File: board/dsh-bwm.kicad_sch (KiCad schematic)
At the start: 17 parts, among them IC2 MAX485CSA+T, K1 833H-1C-C-24VDC, K2 833H-1C-C-24VDC, K3 833H-1C-C-24VDC, K4 833H-1C-C-24VDC, Q1 IRLB8721PBF, SW1 BOOTSEL, SW2 SW_DIP_x09, U1 RP2040_Stamp

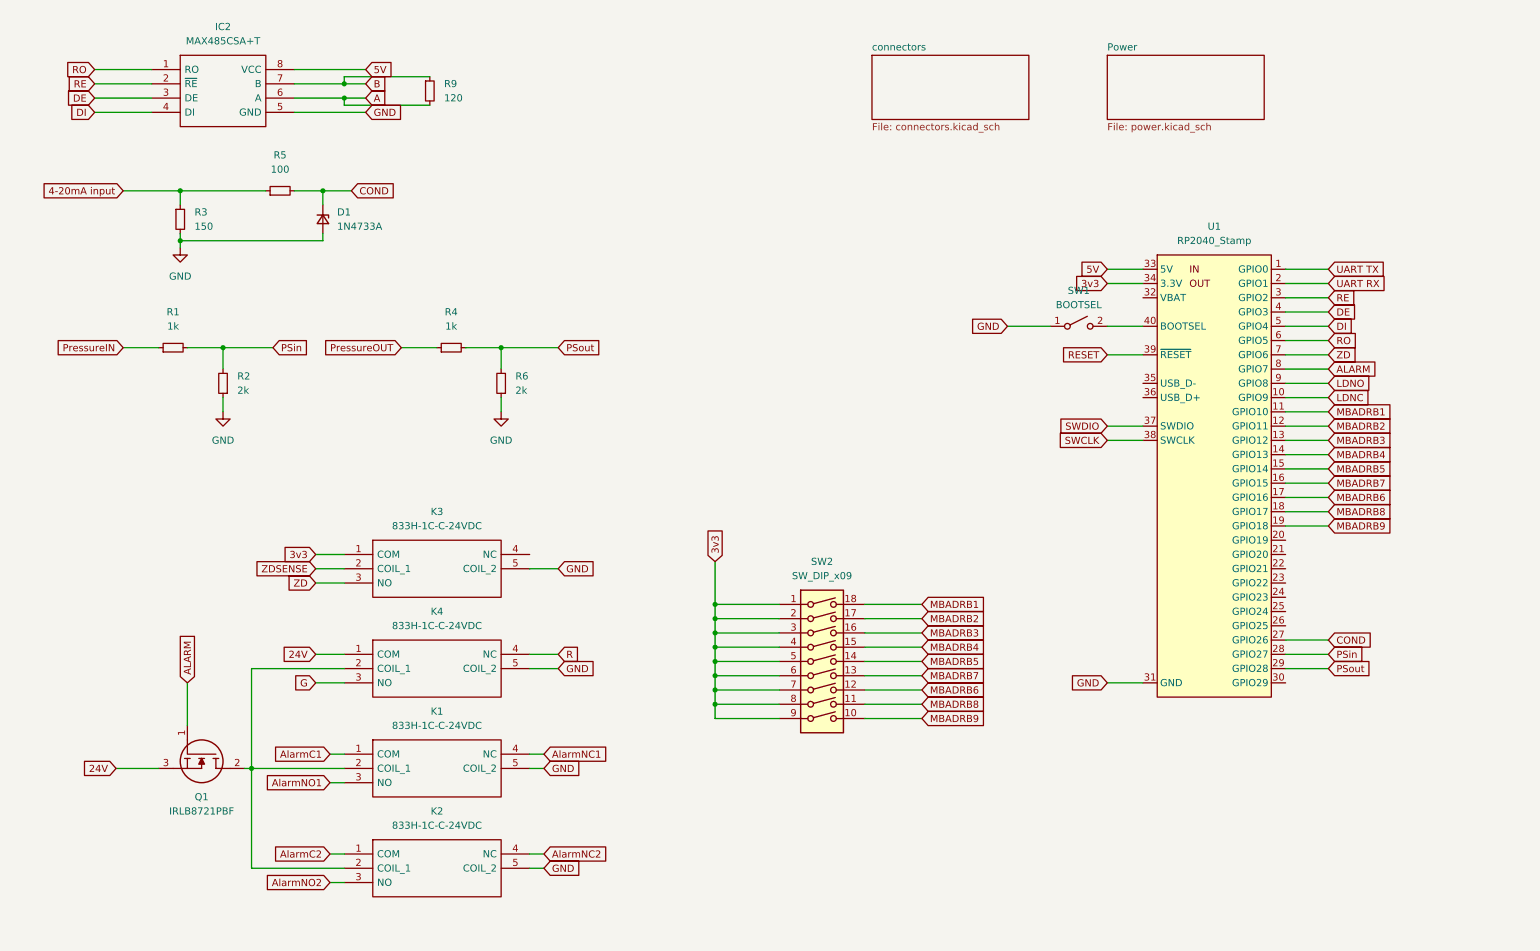
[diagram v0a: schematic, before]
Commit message: TPs, vias, some comments on board, fml
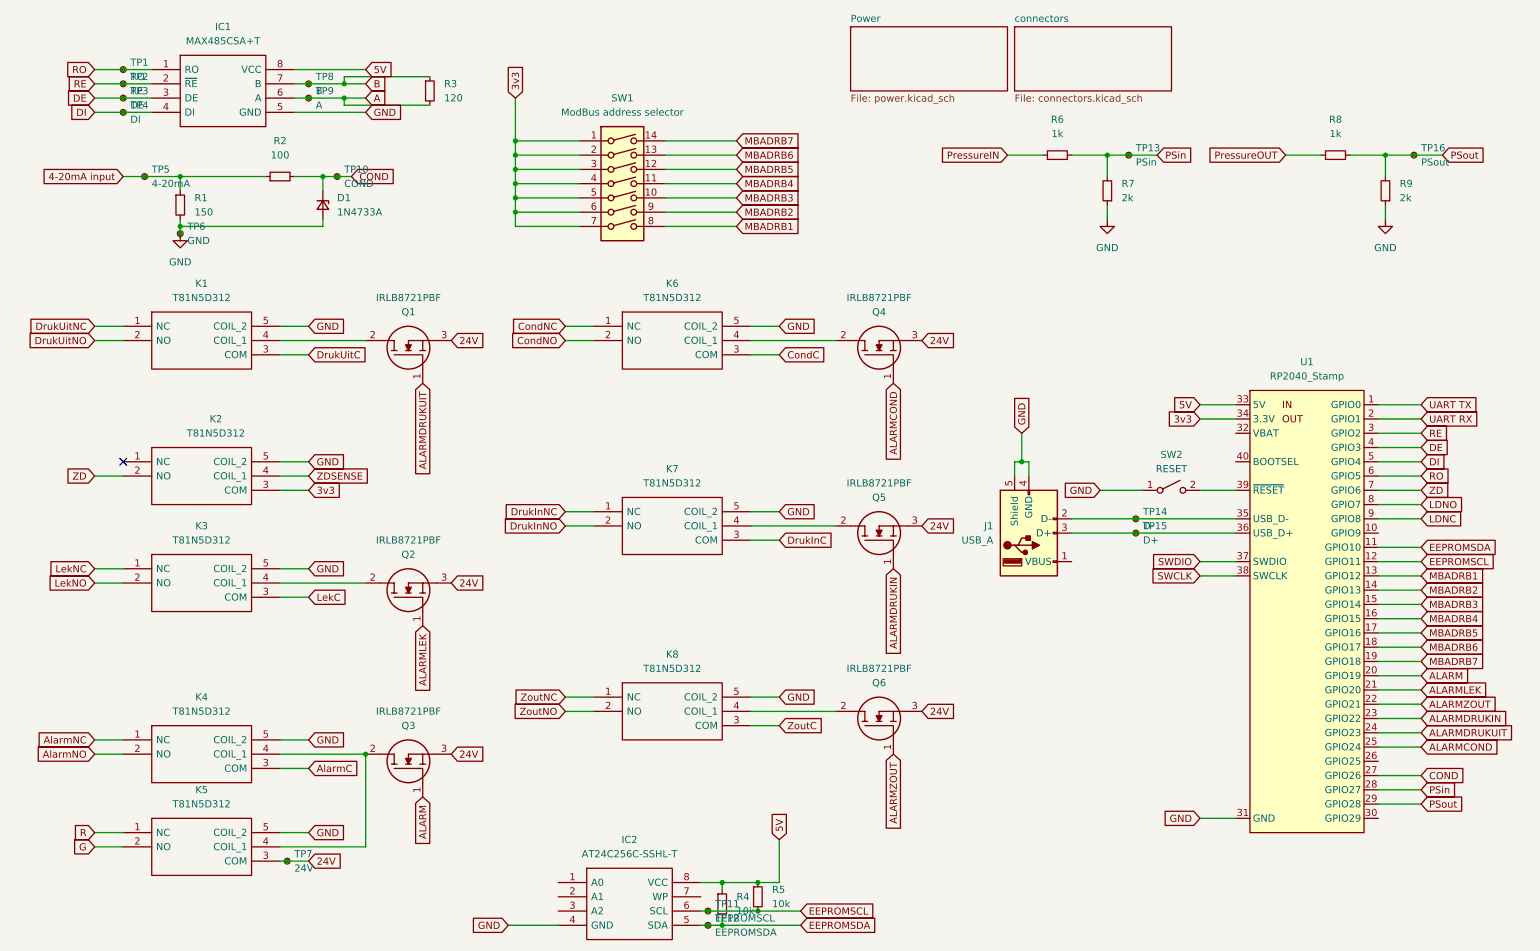
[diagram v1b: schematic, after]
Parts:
- removed R1: 1k, Resistor_SMD:R_0805_2012Metric, symbol Device:R_Small
- removed R2: 2k, Resistor_SMD:R_0805_2012Metric, symbol Device:R_Small
- removed SW1: BOOTSEL, Button_Switch_SMD:SW_SPST_B3U-1000P, symbol Switch:SW_SPST
- added IC2: AT24C256C-SSHL-T, SamacSys_Parts:SOIC127P600X175-8N, symbol SamacSys_Parts:AT24C256C-SSHL-T
- added J1: USB_A, Connector_USB:USB_A_Molex_105057_Vertical, symbol Connector:USB_A
- added K1, K6, K7, K8: T81N5D312, SamacSys_Parts:T81H5D31212, symbol SamacSys_Parts:T81N5D312-05
- added Q1, Q2, Q4, Q5, Q6: IRLB8721PBF, SamacSys_Parts:TO254P483X1016X1994-3P, symbol SamacSys_Parts:IRLB8721PBF
- added R5: 10k, Resistor_SMD:R_0805_2012Metric, symbol Device:R_Small
- added R7, R9: 2k, Resistor_SMD:R_0805_2012Metric, symbol Device:R_Small
- added R8: 1k, Resistor_SMD:R_0805_2012Metric, symbol Device:R_Small
- added SW2: RESET, Button_Switch_SMD:SW_SPST_B3U-1000P, symbol Switch:SW_SPST
- added TP1: RO, TestPoint:TestPoint_Pad_D1.5mm, symbol Connector:TestPoint_Small
- added TP10: COND, TestPoint:TestPoint_Pad_D1.5mm, symbol Connector:TestPoint_Small
- added TP11: EEPROMSCL, TestPoint:TestPoint_Pad_D1.5mm, symbol Connector:TestPoint_Small
- added TP12: EEPROMSDA, TestPoint:TestPoint_Pad_D1.5mm, symbol Connector:TestPoint_Small
- added TP13: PSin, TestPoint:TestPoint_Pad_D1.5mm, symbol Connector:TestPoint_Small
- added TP14: D-, TestPoint:TestPoint_Pad_D1.5mm, symbol Connector:TestPoint_Small
- added TP15: D+, TestPoint:TestPoint_Pad_D1.5mm, symbol Connector:TestPoint_Small
- added TP16: PSout, TestPoint:TestPoint_Pad_D1.5mm, symbol Connector:TestPoint_Small
- added TP2: RE, TestPoint:TestPoint_Pad_D1.5mm, symbol Connector:TestPoint_Small
- added TP3: DE, TestPoint:TestPoint_Pad_D1.5mm, symbol Connector:TestPoint_Small
- added TP4: DI, TestPoint:TestPoint_Pad_D1.5mm, symbol Connector:TestPoint_Small
- added TP5: 4-20mA, TestPoint:TestPoint_Pad_D1.5mm, symbol Connector:TestPoint_Small
- added TP6: GND, TestPoint:TestPoint_Pad_D1.5mm, symbol Connector:TestPoint_Small
- added TP7: 24V, TestPoint:TestPoint_Pad_D1.5mm, symbol Connector:TestPoint_Small
- added TP8: B, TestPoint:TestPoint_Pad_D1.5mm, symbol Connector:TestPoint_Small
- added TP9: A, TestPoint:TestPoint_Pad_D1.5mm, symbol Connector:TestPoint_Small
- K2: renamed from K3; value 833H-1C-C-24VDC -> T81N5D312; footprint SamacSys_Parts:833H1CC24VDC -> SamacSys_Parts:T81H5D31212; symbol SamacSys_Parts:833H-1C-C-24VDC -> SamacSys_Parts:T81N5D312-05; Arrow Part Number (none) -> T81N5D312-05; Arrow Price/Stock (none) -> https://www.arrow.com/en/products/t81n5d312-05/te-connectiv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; Height 15.5 -> 11.7; Manufacturer_Name Song Chuan -> TE Connectivity; Manufacturer_Part_Number 833H-1C-C-24VDC -> T81N5D312-05; Mouser Part Number 893-833H-1C-C-24VDC -> 655-T81N5D312-05; Mouser Price/Stock https://www.mouser.co.uk/ProductDetail/Song-Chuan/833H-1C-C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 -> https://www.mouser.co.uk/ProductDetail/TE-Connectivity-PB/T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
- K3: renamed from K1; value 833H-1C-C-24VDC -> T81N5D312; footprint SamacSys_Parts:833H1CC24VDC -> SamacSys_Parts:T81H5D31212; symbol SamacSys_Parts:833H-1C-C-24VDC -> SamacSys_Parts:T81N5D312-05; Arrow Part Number (none) -> T81N5D312-05; Arrow Price/Stock (none) -> https://www.arrow.com/en/products/t81n5d312-05/te-connectiv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; Height 15.5 -> 11.7; Manufacturer_Name Song Chuan -> TE Connectivity; Manufacturer_Part_Number 833H-1C-C-24VDC -> T81N5D312-05; Mouser Part Number 893-833H-1C-C-24VDC -> 655-T81N5D312-05; Mouser Price/Stock https://www.mouser.co.uk/ProductDetail/Song-Chuan/833H-1C-C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 -> https://www.mouser.co.uk/ProductDetail/TE-Connectivity-PB/T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
- K4: renamed from K2; value 833H-1C-C-24VDC -> T81N5D312; footprint SamacSys_Parts:833H1CC24VDC -> SamacSys_Parts:T81H5D31212; symbol SamacSys_Parts:833H-1C-C-24VDC -> SamacSys_Parts:T81N5D312-05; Arrow Part Number (none) -> T81N5D312-05; Arrow Price/Stock (none) -> https://www.arrow.com/en/products/t81n5d312-05/te-connectiv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; Height 15.5 -> 11.7; Manufacturer_Name Song Chuan -> TE Connectivity; Manufacturer_Part_Number 833H-1C-C-24VDC -> T81N5D312-05; Mouser Part Number 893-833H-1C-C-24VDC -> 655-T81N5D312-05; Mouser Price/Stock https://www.mouser.co.uk/ProductDetail/Song-Chuan/833H-1C-C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 -> https://www.mouser.co.uk/ProductDetail/TE-Connectivity-PB/T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
- K5: renamed from K4; value 833H-1C-C-24VDC -> T81N5D312; footprint SamacSys_Parts:833H1CC24VDC -> SamacSys_Parts:T81H5D31212; symbol SamacSys_Parts:833H-1C-C-24VDC -> SamacSys_Parts:T81N5D312-05; Arrow Part Number (none) -> T81N5D312-05; Arrow Price/Stock (none) -> https://www.arrow.com/en/products/t81n5d312-05/te-connectiv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; Height 15.5 -> 11.7; Manufacturer_Name Song Chuan -> TE Connectivity; Manufacturer_Part_Number 833H-1C-C-24VDC -> T81N5D312-05; Mouser Part Number 893-833H-1C-C-24VDC -> 655-T81N5D312-05; Mouser Price/Stock https://www.mouser.co.uk/ProductDetail/Song-Chuan/833H-1C-C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 -> https://www.mouser.co.uk/ProductDetail/TE-Connectivity-PB/T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
- R4: value 1k -> 10k; JLC (none) -> 0402WGF1500TCE
- R6: value 2k -> 1k
- SW1: renamed from SW2; value SW_DIP_x09 -> ModBus address selector; footprint Button_Switch_THT:SW_DIP_SPSTx09_Slide_6.7x24.42mm_W7.62mm_P2.54mm_LowProfile -> Button_Switch_THT:SW_DIP_SPSTx07_Slide_6.7x19.34mm_W7.62mm_P2.54mm_LowProfile; symbol Switch:SW_DIP_x09 -> Switch:SW_DIP_x07
- renumbered IC2 to IC1, Q1 to Q3, R3 to R1, R5 to R2, R9 to R3
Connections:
- net 24V: now also K5.3 (COM), Q1.3, Q2.3, Q4.3, Q5.3, Q6.3, TP7.1; no longer K5.1 (COM)
- net 3v3: now also K2.3 (COM); no longer K2.1 (COM), SW1.8, SW1.9
- net 4-20mA input: now also TP5.1
- net 5V: now also R4.1, IC2.8 (VCC), R5.1
- net A: now also TP9.1
- net ALARM: now also U1.20 (GPIO19); no longer U1.8 (GPIO7)
- net B: now also TP8.1
- net COND: now also TP10.1
- net DE: now also TP3.1
- net DI: now also TP4.1
- net G: now also K5.2 (NO); no longer K5.3 (NO)
- net GND: now also IC2.4 (GND), J1.4 (GND), J1.5 (Shield), K1.5 (COIL_2), K6.5 (COIL_2), K7.5 (COIL_2), K8.5 (COIL_2), R7.1, R9.1, SW2.1 (A), TP6.1; no longer R6.1
- net LDNC: now also U1.9 (GPIO8); no longer U1.10 (GPIO9)
- net LDNO: now also U1.8 (GPIO7); no longer U1.9 (GPIO8)
- net MBADRB1: now also SW1.8, U1.13 (GPIO12); no longer SW1.18, U1.11 (GPIO10)
- net MBADRB2: now also SW1.9, U1.14 (GPIO13); no longer SW1.17, U1.12 (GPIO11)
- net MBADRB3: now also SW1.10, U1.15 (GPIO14); no longer SW1.16, U1.13 (GPIO12)
- net MBADRB4: now also SW1.11, U1.16 (GPIO15); no longer SW1.15, U1.14 (GPIO13)
- net MBADRB5: now also SW1.12, U1.17 (GPIO16); no longer SW1.14, U1.15 (GPIO14)
- net MBADRB6: now also SW1.13, U1.18 (GPIO17); no longer SW1.12, U1.17 (GPIO16)
- net MBADRB7: now also SW1.14, U1.19 (GPIO18); no longer SW1.13, U1.16 (GPIO15)
- net PSin: now also R6.2, R7.2, TP13.1
- net PSout: now also R8.2, R9.2, TP16.1; no longer R4.2, R6.2
- net PressureIN: now also R6.1
- net PressureOUT: now also R8.1; no longer R4.1
- net R: now also K5.1 (NC); no longer K5.4 (NC)
- net RE: now also TP2.1
- net RO: now also TP1.1
- net ZD: now also K2.2 (NO); no longer K2.3 (NO)
- net ZDSENSE: now also K2.4 (COIL_1); no longer K2.2 (COIL_1)
- net ALARMLEK: now reaches U1.21 (GPIO20)
- net ALARMLEK: now also Q2.1
- net ALARMZOUT: now reaches U1.22 (GPIO21)
- net ALARMZOUT: now also Q6.1
- net ALARMDRUKIN: now reaches U1.23 (GPIO22)
- net ALARMDRUKIN: now also Q5.1
- net ALARMDRUKUIT: now reaches U1.24 (GPIO23)
- net ALARMDRUKUIT: now also Q1.1
- net ALARMCOND: now reaches U1.25 (GPIO24)
- net ALARMCOND: now also Q4.1
- net at U1.35 (USB_D-): now also J1.2 (D-), TP14.1
- net at U1.36 (USB_D+): now also J1.3 (D+), TP15.1
- net AlarmC1 renamed LekNC
- net AlarmC2 renamed AlarmNC
- net AlarmNC1: no longer names the net of K3.4 (COIL_1)
- net AlarmNC1: now also Q2.2
- net AlarmNC2: no longer names the net of K4.4 (COIL_1)
- net AlarmNC2: now also K5.4 (COIL_1), Q3.2
- net AlarmNO1 renamed LekC
- net AlarmNO2 renamed AlarmC
- removed net MBADRB8: SW1.11, U1.18 (GPIO17)
- removed net MBADRB9: SW1.10, U1.19 (GPIO18)
- net RESET: no longer names the net of U1.39 (~{RESET})
- net RESET: now also SW2.2 (B)
- new net: K6.4 (COIL_1), Q4.2
- new net: K8.4 (COIL_1), Q6.2
- new net: K1.4 (COIL_1), Q1.2
- new net: K7.4 (COIL_1), Q5.2
- new net AlarmNO: K4.2 (NO)
- new net CondC: K6.3 (COM)
- new net CondNC: K6.1 (NC)
- new net CondNO: K6.2 (NO)
- new net DrukInC: K7.3 (COM)
- new net DrukInNC: K7.1 (NC)
- new net DrukInNO: K7.2 (NO)
- new net DrukUitC: K1.3 (COM)
- new net DrukUitNC: K1.1 (NC)
- new net DrukUitNO: K1.2 (NO)
- new net EEPROMSCL: IC2.6 (SCL), R5.2, TP11.1, U1.12 (GPIO11)
- new net EEPROMSDA: IC2.5 (SDA), R4.2, TP12.1, U1.11 (GPIO10)
- new net LekNO: K3.2 (NO)
- new net ZoutC: K8.3 (COM)
- new net ZoutNC: K8.1 (NC)
- new net ZoutNO: K8.2 (NO)
- no-connect marks 0 -> 1
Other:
- moved on the sheet: D1, K2, K3, K4, K5, Q3, R1, R2, U1
